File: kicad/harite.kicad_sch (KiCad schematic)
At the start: 76 parts, among them J1 Cirque Connector, J2 Cirque Connector, U1 RP2040_Zero, U2 RP2040_Zero

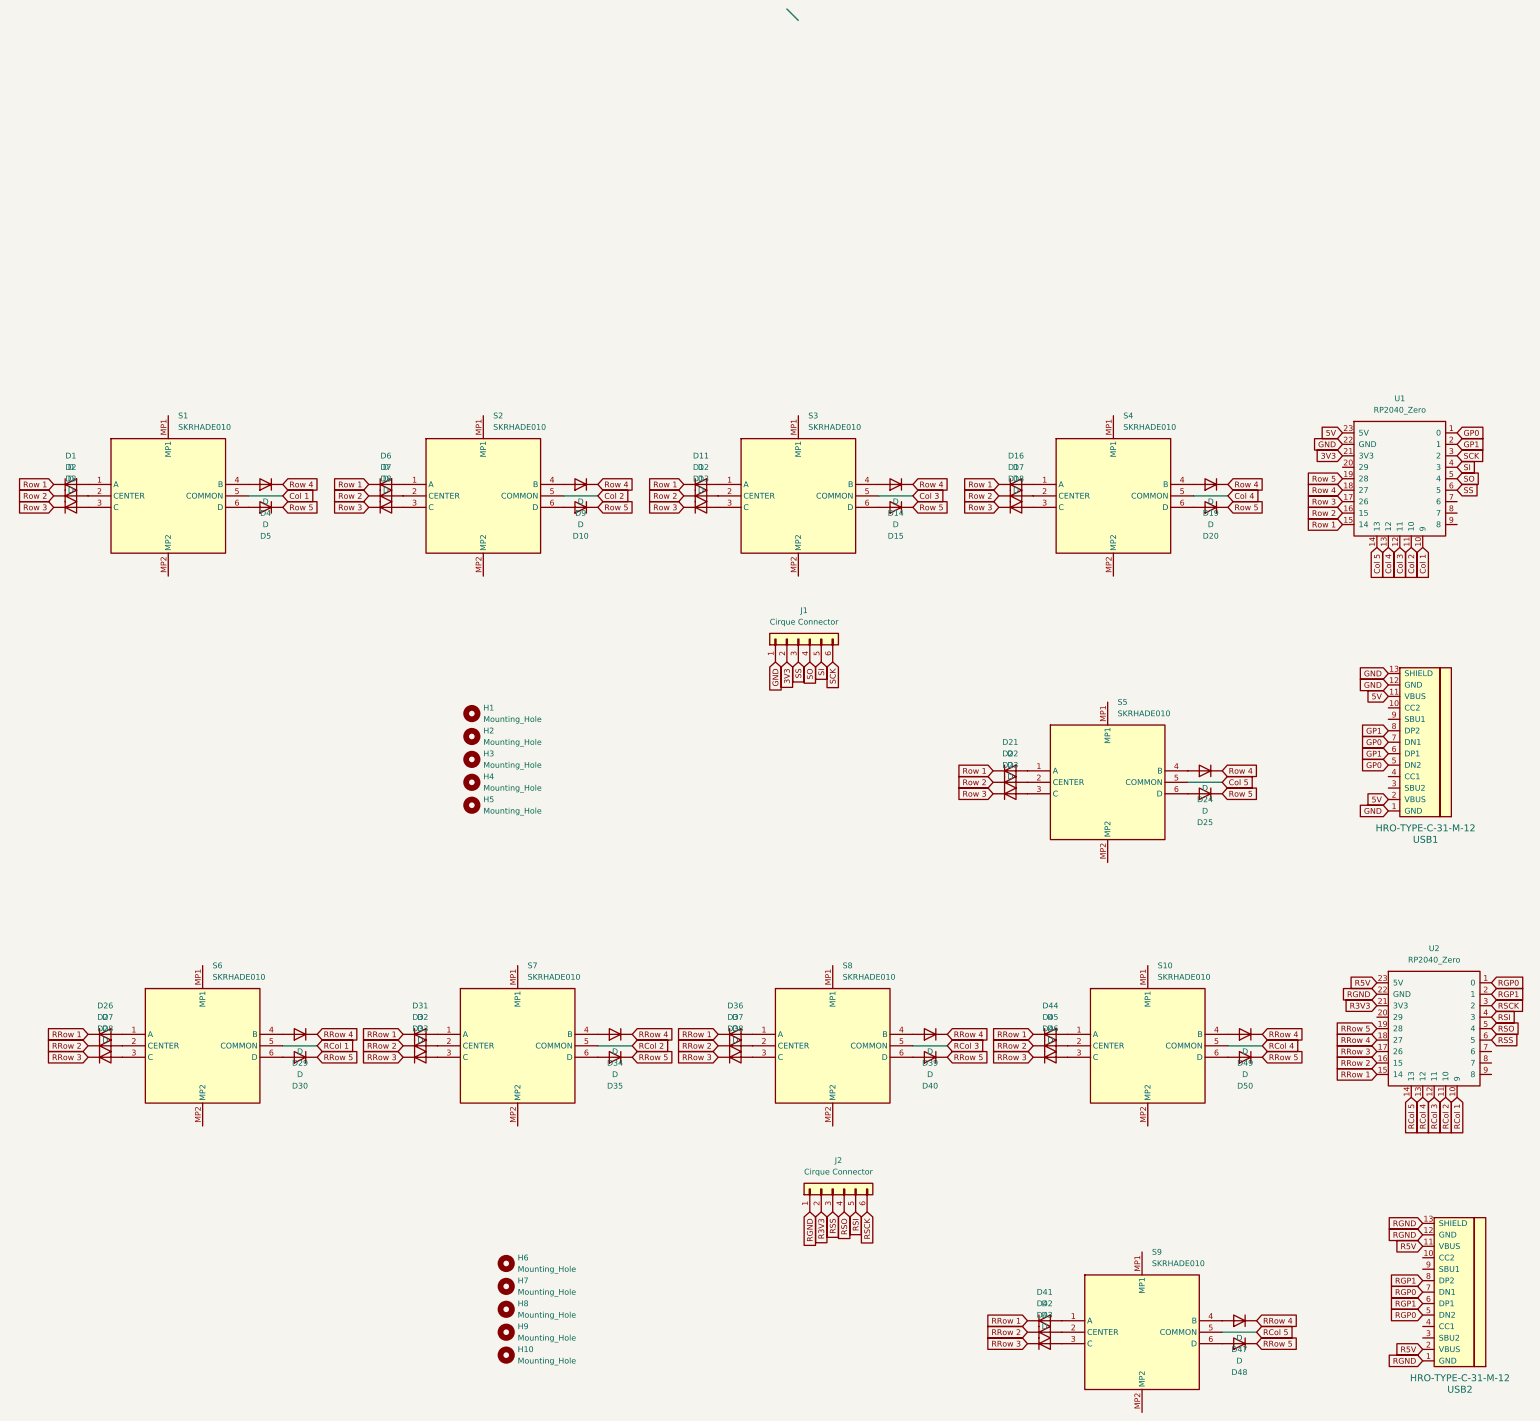
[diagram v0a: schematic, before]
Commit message: basic schematic
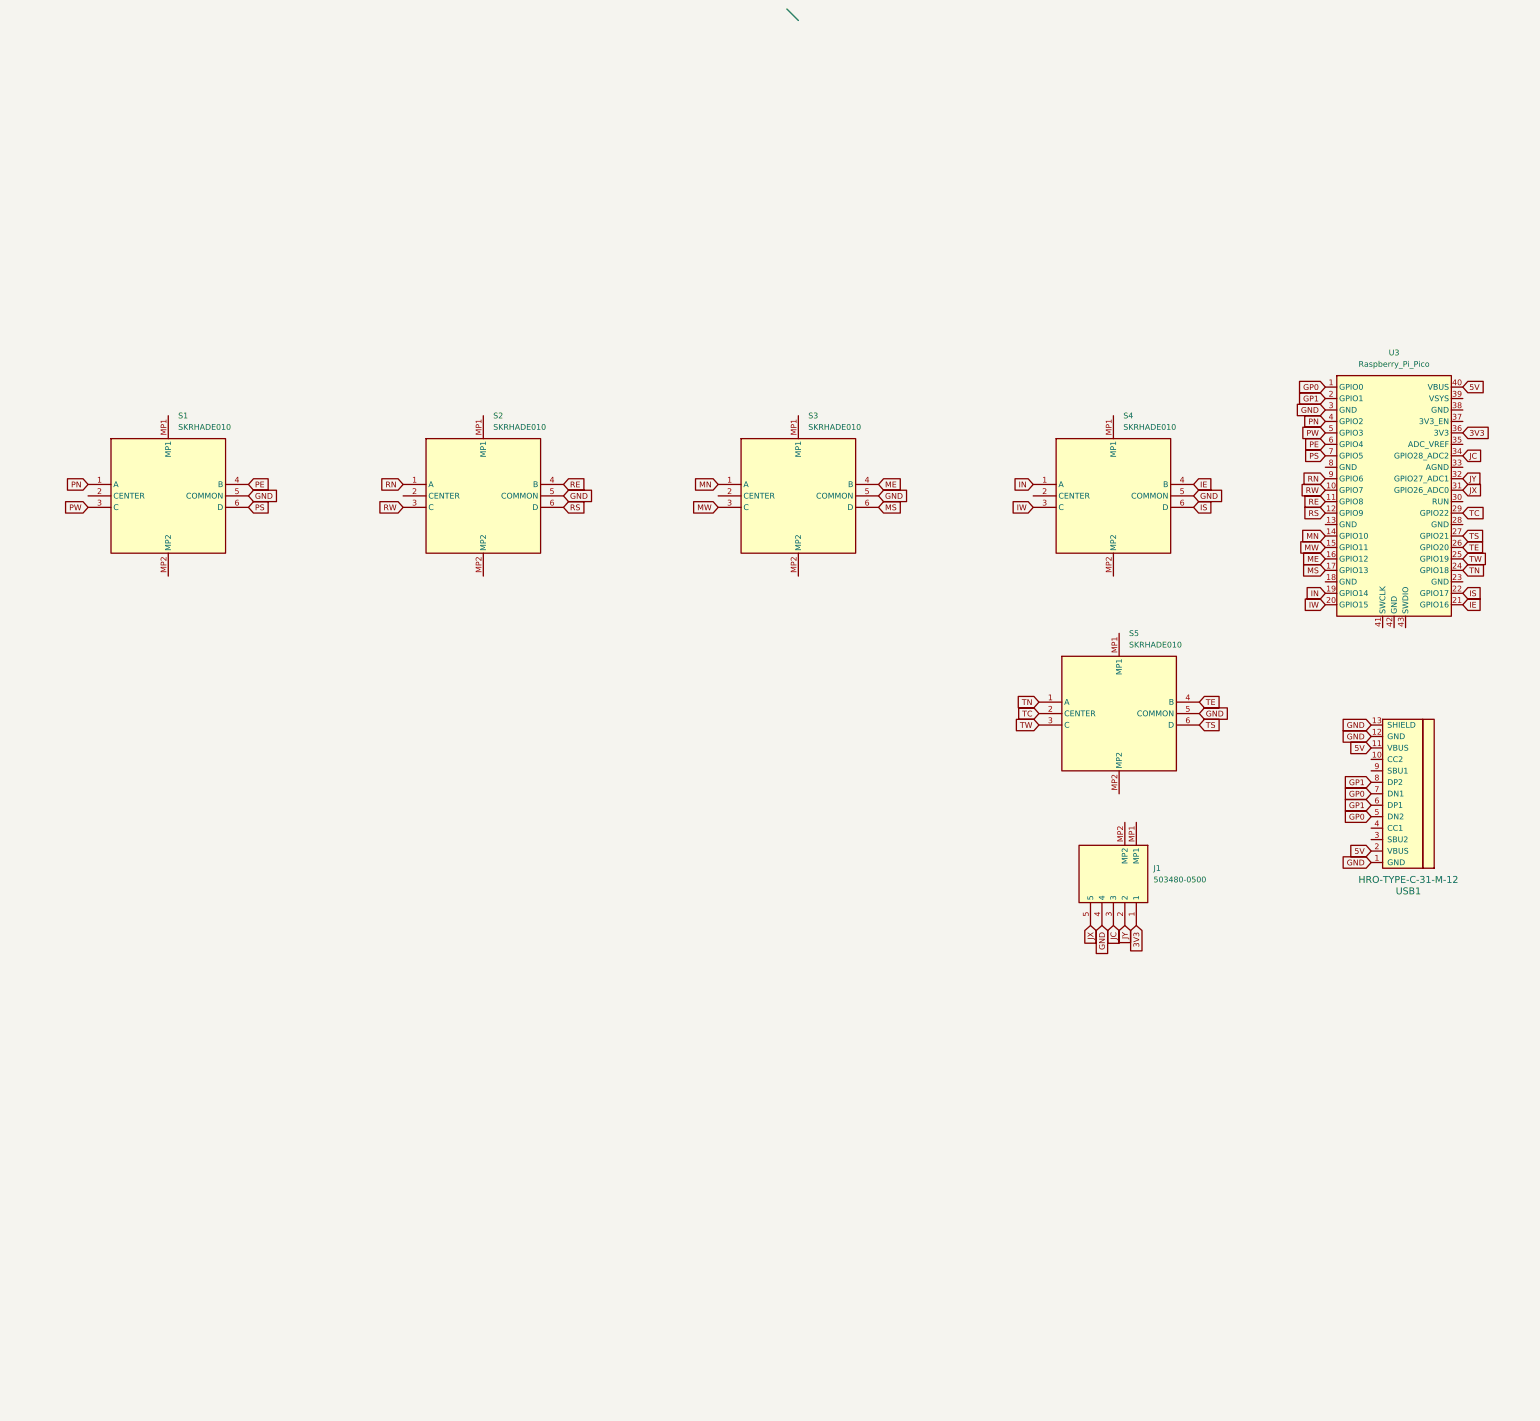
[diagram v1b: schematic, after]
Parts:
- removed D1, D10, D11, D12, D13, D14, D15, D16, D17, D18, D19, D2, D20, D21, D22, D23, D24, D25, D26, D27, D28, D29, D3, D30, D31, D32, D33, D34, D35, D36, D37, D38, D39, D4, D40, D41, D42, D43, D44, D45, D46, D47, D48, D49, D5, D50, D6, D7, D8, D9: D, ScottoKeebs_Components:Diode_SOD-123, symbol Device:D
- removed H1, H10, H2, H3, H4, H5, H6, H7, H8, H9: Mounting_Hole, MountingHole:MountingHole_2.2mm_M2_Pad_Via, symbol ScottoKeebs:Placeholder_Mounting_Hole
- removed J1, J2: Cirque Connector, footprints:Cirque-connector, symbol Connector_Generic:Conn_01x06
- removed S10, S6, S7, S8, S9: SKRHADE010, footprints:SKRHADE, symbol SKRHADE010:SKRHADE010
- removed U1, U2: RP2040_Zero, ScottoKeebs_MCU:RP2040_Zero, symbol ScottoKeebs:MCU_RP2040_Zero
- removed USB2: HRO-TYPE-C-31-M-12, footprints:HRO-TYPE-C-31-M-12, symbol USBType-C:HRO-TYPE-C-31-M-12
- added J1: 503480-0500, 5034800500, symbol 503480-0500:503480-0500
- added U3: Raspberry_Pi_Pico, ScottoKeebs_MCU:Raspberry_Pi_Pico, symbol ScottoKeebs:MCU_Raspberry_Pi_Pico
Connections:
- net Col 1 is gone; now on net GND: S1.5 (COMMON)
- net Col 2 is gone; now on net GND: S2.5 (COMMON)
- net Col 3 is gone; now on net GND: S3.5 (COMMON)
- net Col 4 is gone; now on net GND: S4.5 (COMMON)
- net Col 5 is gone; now on net GND: S5.5 (COMMON)
- net 3V3: now also J1.1, U3.36 (3V3)
- net 5V: now also U3.40 (VBUS)
- net GND: now also J1.4, U3.3 (GND)
- net GP0: now also U3.1 (GPIO0)
- net GP1: now also U3.2 (GPIO1)
- net TW: now reaches S5.3 (C)
- net TW: now also U3.25 (GPIO19)
- net PS: now reaches S1.6 (D)
- net PS: now also U3.7 (GPIO5)
- net PN: now reaches S1.1 (A)
- net PN: now also U3.4 (GPIO2)
- net PW: now reaches S1.3 (C)
- net PW: now also U3.5 (GPIO3)
- net PE: now reaches S1.4 (B)
- net PE: now also U3.6 (GPIO4)
- net IE: now reaches S4.4 (B)
- net IE: now also U3.21 (GPIO16)
- net TC: now reaches S5.2 (CENTER)
- net TC: now also U3.29 (GPIO22)
- net RN: now reaches S2.1 (A)
- net RN: now also U3.9 (GPIO6)
- net RW: now reaches S2.3 (C)
- net RW: now also U3.10 (GPIO7)
- net RE: now reaches S2.4 (B)
- net RE: now also U3.11 (GPIO8)
- net RS: now reaches S2.6 (D)
- net RS: now also U3.12 (GPIO9)
- net TN: now reaches S5.1 (A)
- net TN: now also U3.24 (GPIO18)
- net TE: now reaches S5.4 (B)
- net TE: now also U3.26 (GPIO20)
- net TS: now reaches S5.6 (D)
- net TS: now also U3.27 (GPIO21)
- net MW: now reaches S3.3 (C)
- net MW: now also U3.15 (GPIO11)
- net MS: now reaches S3.6 (D)
- net MS: now also U3.17 (GPIO13)
- net MN: now reaches S3.1 (A)
- net MN: now also U3.14 (GPIO10)
- net ME: now reaches S3.4 (B)
- net ME: now also U3.16 (GPIO12)
- net IN: now reaches S4.1 (A)
- net IN: now also U3.19 (GPIO14)
- net IW: now reaches S4.3 (C)
- net IW: now also U3.20 (GPIO15)
- net IS: now reaches S4.6 (D)
- net IS: now also U3.22 (GPIO17)
- new net JC: J1.3, U3.34 (GPIO28_ADC2)
- new net JX: J1.5, U3.31 (GPIO26_ADC0)
- new net JY: J1.2, U3.32 (GPIO27_ADC1)
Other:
- moved on the sheet: S5, USB1
